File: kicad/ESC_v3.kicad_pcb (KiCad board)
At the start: 6 copper layers, 50 x 50 mm, 165 parts, among them J1 Conn_01x05_Pin, J2 Conn_01x05_Pin, J4 Conn_01x06_Pin, J6 Conn_01x06_Pin, J7 Conn_01x02_Pin, J8 Conn_01x04_Pin, J9 Conn_01x02_Pin, Q1 RH6L040BGTB1, Q10 RH6L040BGTB1, Q11 RH6L040BGTB1, Q12 RH6L040BGTB1, Q2 RH6L040BGTB1, Q3 RH6L040BGTB1, Q4 RH6L040BGTB1, Q5 RH6L040BGTB1, Q6 RH6L040BGTB1, Q7 RH6L040BGTB1, Q8 RH6L040BGTB1, Q9 RH6L040BGTB1, SW2 SW_Nidec_CAS-120A1, U1 L6387, U10 BD4104, U11 AMS1117-5.0, U12 ACS711xEXLT-15AB, U13 LM2937xMP, U14 MCP9700x-ETT, U15 MAX40200AUK, U16 AS5048A, U19 STM32G431CBUx, U2 L6387, U3 L6387, U4 L6387, U5 L6387, U6 L6387, U7 AMS1117-3.3, U8 ACS711xEXLT-15AB, U9 ACS711xEXLT-15AB

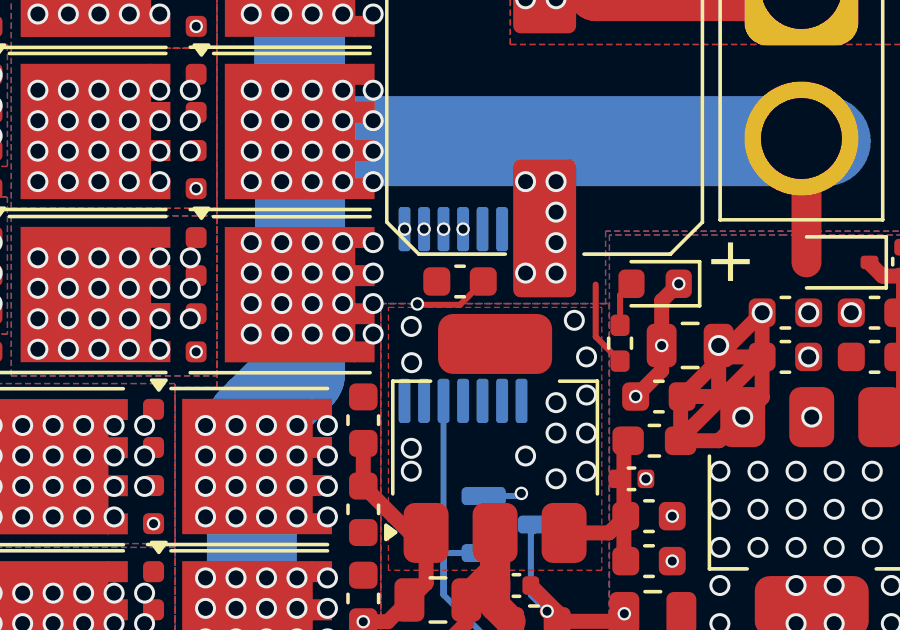
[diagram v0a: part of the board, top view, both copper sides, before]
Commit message: a
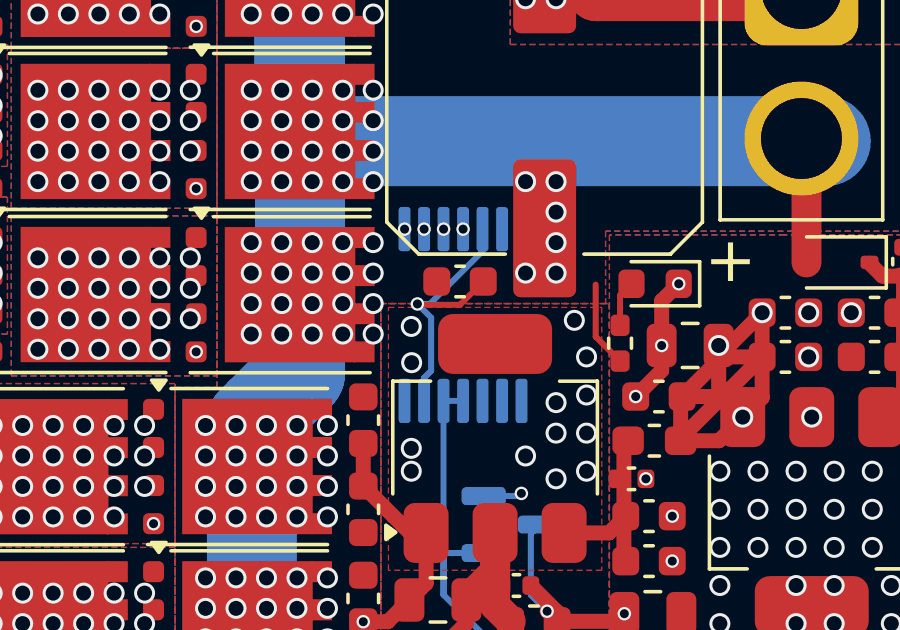
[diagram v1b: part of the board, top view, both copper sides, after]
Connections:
- U16 pad 11: unconnected-(U16-VDD5V-Pad11) -> +3.3V
- U16 pad 13: unconnected-(U16-GND-Pad13) -> GND
- U16 pad 5: unconnected-(U16-TEST-Pad5) -> GND
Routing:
- net GND: track 107.2 -> 114.4 mm
- net +3.3V: track 67.3 -> 68.0 mm
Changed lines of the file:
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@@
 	(net 118 "unconnected-(U10-SPLIT-Pad5)")
 	(net 119 "unconnected-(U16-TEST-Pad10)")
-	(net 120 "unconnected-(U16-GND-Pad13)")
-	(net 121 "unconnected-(U16-TEST-Pad7)")
-	(net 122 "unconnected-(U16-PWM-Pad14)")
-	(net 123 "unconnected-(U16-VDD5V-Pad11)")
-	(net 124 "unconnected-(U16-TEST-Pad6)")
-	(net 125 "unconnected-(U16-TEST-Pad8)")
-	(net 126 "unconnected-(U16-TEST-Pad5)")
-	(net 127 "unconnected-(U16-TEST-Pad9)")
-	(net 128 "Net-(R43-Pad2)")
+	(net 120 "unconnected-(U16-TEST-Pad7)")
+	(net 121 "unconnected-(U16-PWM-Pad14)")
+	(net 122 "unconnected-(U16-TEST-Pad6)")
+	(net 123 "unconnected-(U16-TEST-Pad8)")
+	(net 124 "unconnected-(U16-TEST-Pad9)")
+	(net 125 "Net-(R43-Pad2)")
 	(footprint "Resistor_SMD:R_2010_5025Metric_Pad1.40x2.65mm_HandSolder"
 		(layer "F.Cu")
@@
 			(size 1 1)
 			(layers "F.Cu" "F.Mask")
-			(net 128 "Net-(R43-Pad2)")
+			(net 125 "Net-(R43-Pad2)")
 			(pinfunction "1")
 			(pintype "passive")
@@
 			(layers "F.Cu" "F.Mask" "F.Paste")
 			(roundrect_rratio 0.25)
-			(net 128 "Net-(R43-Pad2)")
+			(net 125 "Net-(R43-Pad2)")
 			(pintype "passive")
 		)
@@
 			(layers "B.Cu" "B.Mask" "B.Paste")
 			(roundrect_rratio 0.25)
-			(net 126 "unconnected-(U16-TEST-Pad5)")
+			(net 107 "GND")
 			(pinfunction "TEST")
 			(pintype "passive")
@@
 			(layers "B.Cu" "B.Mask" "B.Paste")
 			(roundrect_rratio 0.25)
-			(net 124 "unconnected-(U16-TEST-Pad6)")
+			(net 122 "unconnected-(U16-TEST-Pad6)")
 			(pinfunction "TEST")
 			(pintype "passive")
@@
 			(layers "B.Cu" "B.Mask" "B.Paste")
 			(roundrect_rratio 0.25)
-			(net 121 "unconnected-(U16-TEST-Pad7)")
+			(net 120 "unconnected-(U16-TEST-Pad7)")
 			(pinfunction "TEST")
 			(pintype "passive")
@@
 			(layers "B.Cu" "B.Mask" "B.Paste")
 			(roundrect_rratio 0.25)
-			(net 125 "unconnected-(U16-TEST-Pad8)")
+			(net 123 "unconnected-(U16-TEST-Pad8)")
 			(pinfunction "TEST")
 			(pintype "passive")
@@
 			(layers "B.Cu" "B.Mask" "B.Paste")
 			(roundrect_rratio 0.25)
-			(net 127 "unconnected-(U16-TEST-Pad9)")
+			(net 124 "unconnected-(U16-TEST-Pad9)")
 			(pinfunction "TEST")
 			(pintype "passive")
@@
 			(layers "B.Cu" "B.Mask" "B.Paste")
 			(roundrect_rratio 0.25)
-			(net 123 "unconnected-(U16-VDD5V-Pad11)")
+			(net 12 "+3.3V")
 			(pinfunction "VDD5V")
 			(pintype "power_in")
@@
 			(layers "B.Cu" "B.Mask" "B.Paste")
 			(roundrect_rratio 0.25)
-			(net 120 "unconnected-(U16-GND-Pad13)")
+			(net 107 "GND")
 			(pinfunction "GND")
 			(pintype "power_in")
@@
 			(layers "B.Cu" "B.Mask" "B.Paste")
 			(roundrect_rratio 0.25)
-			(net 122 "unconnected-(U16-PWM-Pad14)")
+			(net 121 "unconnected-(U16-PWM-Pad14)")
 			(pinfunction "PWM")
 			(pintype "output")
@@
 	)
 	(segment
+		(start 84.7852 73.8555)
+		(end 84.1352 73.8555)
+		(width 0.2)
+		(layer "B.Cu")
+		(net 12)
+	)
+	(segment
 		(start 84.1352 78.928)
 		(end 84.1352 80.3252)
@@
 	)
 	(segment
+		(start 83.4852 73.8555)
+		(end 83.4852 73.087898)
+		(width 0.2)
+		(layer "B.Cu")
+		(net 107)
+	)
+	(segment
 		(start 81.534 83.9484)
 		(end 81.534 81.293)
@@
 	)
 	(segment
+		(start 83.721305 72.851793)
+		(end 83.721305 71.083524)
+		(width 0.2)
+		(layer "B.Cu")
+		(net 107)
+	)
+	(segment
 		(start 87.5857 80.8671)
 		(end 87.0432 80.3246)
@@
 	)
 	(segment
+		(start 85.4352 68.867999)
+		(end 83.678699 70.6245)
+		(width 0.2)
+		(layer "B.Cu")
+		(net 107)
+	)
+	(segment
 		(start 81.534 81.293)
 		(end 81.4578 81.2168)
@@
 	)
 	(segment
+		(start 83.4852 73.087898)
+		(end 83.721305 72.851793)
+		(width 0.2)
+		(layer "B.Cu")
+		(net 107)
+	)
+	(segment
 		(start 55.6862 68.4396)
 		(end 54.628519 68.4396)
@@
 	)
 	(segment
+		(start 83.678699 70.6245)
+		(end 83.262281 70.6245)
+		(width 0.2)
+		(layer "B.Cu")
+		(net 107)
+	)
+	(segment
 		(start 87.0432 80.3246)
 		(end 87.0432 78.2831)
@@
 	)
 	(segment
+		(start 85.4352 68.1305)
+		(end 85.4352 68.867999)
+		(width 0.2)
+		(layer "B.Cu")
+		(net 107)
+	)
+	(segment
+		(start 83.721305 71.083524)
+		(end 83.262281 70.6245)
+		(width 0.2)
+		(layer "B.Cu")
+		(net 107)
+	)
+	(segment
 		(start 71.2242 98.311639)
 		(end 71.2242 97.6969)
@@
 		(width 0.2)
 		(layer "F.Cu")
-		(net 128)
+		(net 125)
 	)
 	(segment
@@
 		(width 0.2)
 		(layer "F.Cu")
-		(net 128)
+		(net 125)
 	)
 	(zone
